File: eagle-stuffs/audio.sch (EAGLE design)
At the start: 23 parts, among them IC1 LM386N-1, IC2 TL084P, IC3 X9C102P, IC4 X9C102P, U1 AT42QT1010SOT23

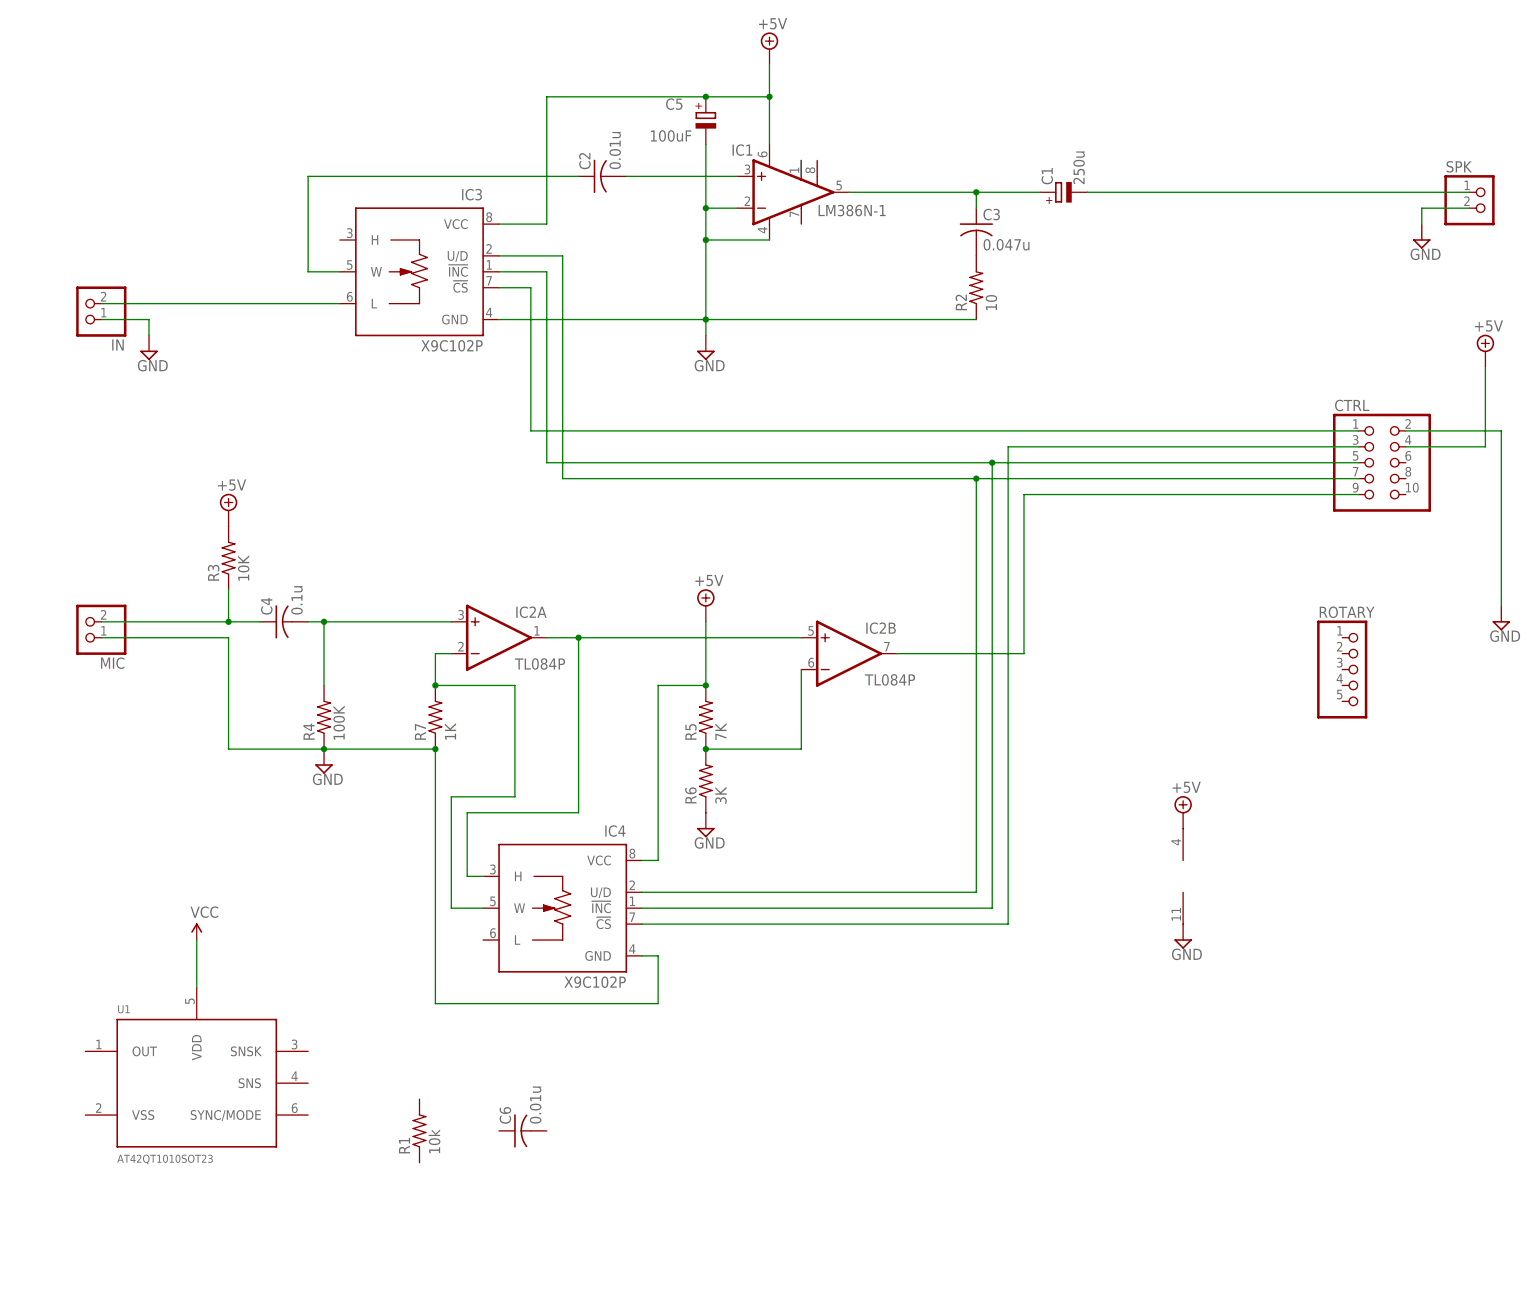
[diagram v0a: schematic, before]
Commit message: Still working on audio…
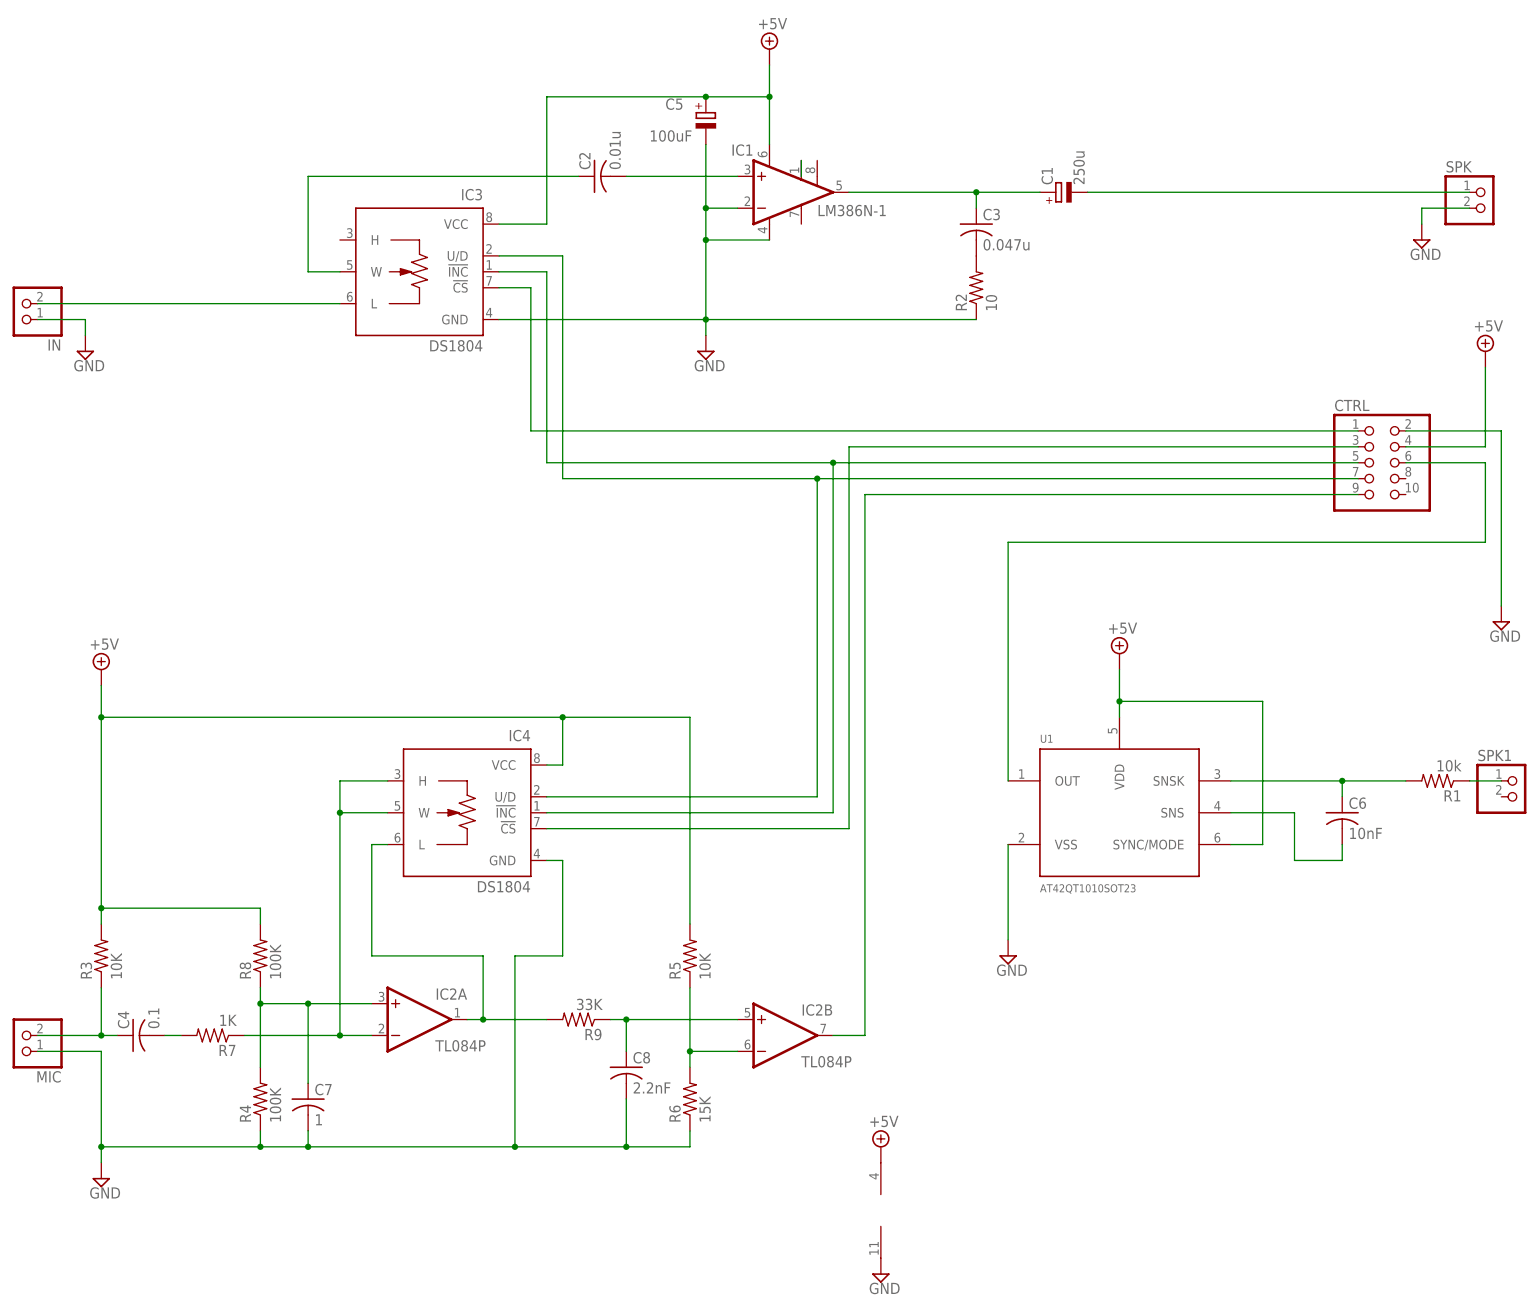
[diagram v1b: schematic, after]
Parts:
- removed ROTARY: (no value), pinhead:PINHD-1X5
- added C7: 1, rcl:C-US025-025X050
- added C8: 2.2nF, rcl:C-US025-025X050
- added R8: 100K, resistor:R-US_0207/10
- added R9: 33K, resistor:R-US_0207/10
- added SPK1: (no value), pinhead:PINHD-1X2
- C4: value 0.1u -> 0.1
- C6: value 0.01u -> 10nF
- IC3, IC4: value X9C102P -> DS1804
- R5: value 7K -> 10K
- R6: value 3K -> 15K
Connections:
- removed net VCC: U1.VDD
- new net N$15: C7.1, IC2A.+IN, R4.2, R8.1
- new net N$16: C6.1, R1.2, U1.SNSK
- new net N$17: C6.2, U1.SNS
- new net N$22: R1.1, SPK1.1
- new net N$24: CTRL.6, U1.OUT
- new net N$8: C4.2, R7.2
- net +5V: now also R8.2, U1.SYNC/MODE, U1.VDD
- net GND: now also C7.2, C8.2, U1.VSS; no longer R7.1
- net N$10: now also IC2A.-IN, IC4.H, IC4.W, R7.1; no longer C4.2, IC2A.+IN, R4.2
- net N$11: now also IC4.L, R9.2; no longer IC2B.+IN, IC4.H
- net N$13: now also C8.1, IC2B.+IN, R9.1; no longer IC2A.-IN, IC4.W, R7.2
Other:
- moved on the sheet: C4, C6, IC2A, IC2B, IC4, IN, MIC, R1, R3, R4, R5, R6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
